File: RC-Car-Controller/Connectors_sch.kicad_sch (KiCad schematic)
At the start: 8 parts, among them J1 Conn_01x02, J4 Conn_01x02, J5 MCU_IF, J6 ANT_IF, J7 2171790001, U2 USBLC6-2SC6

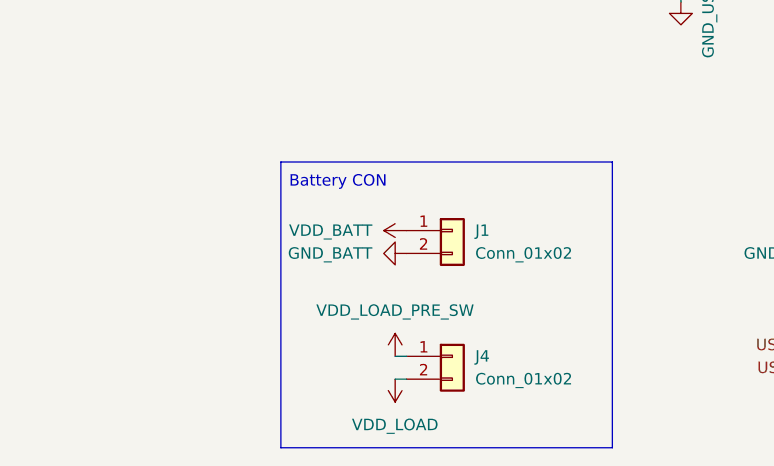
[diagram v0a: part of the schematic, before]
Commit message: Added a switch
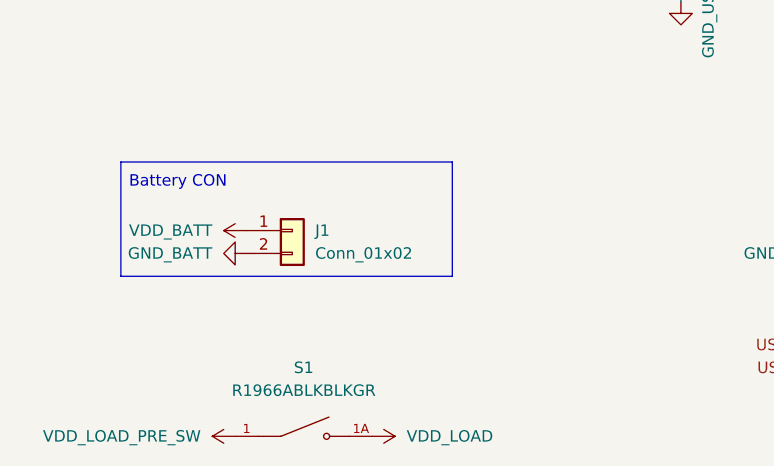
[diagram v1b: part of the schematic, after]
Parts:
- removed J4: Conn_01x02, Connector_JST:JST_XH_B2B-XH-AM_1x02_P2.50mm_Vertical, symbol Connector_Generic:Conn_01x02
- added S1: R1966ABLKBLKGR, R1966ABLKBLKGR:SW_R1966ABLKBLKGR, symbol R1966ABLKBLKGR:R1966ABLKBLKGR
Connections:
- net VDD_LOAD: now also S1.1A
- net VDD_LOAD_PRE_SW: now also S1.1
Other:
- moved on the sheet: J1
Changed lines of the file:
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@@
 		)
 	)
-	(wire
-		(pts
-			(xy 73.66 146.05) (xy 72.39 146.05)
-		)
+	(rectangle
+		(start 41.91 121.92)
+		(end 78.74 134.62)
 		(stroke
 			(width 0)
 			(type default)
 		)
-	)
-	(wire
-		(pts
-			(xy 73.66 143.51) (xy 72.39 143.51)
-		)
-		(stroke
-			(width 0)
-			(type default)
-		)
-	)
-	(rectangle
-		(start 59.69 121.92)
-		(end 96.52 153.67)
-		(stroke
-			(width 0)
-			(type default)
-		)
 		(fill
 			(type none)
@@
 	(text "Battery CON"
 		(exclude_from_sim no)
-		(at 66.04 124.206 0)
+		(at 48.26 124.206 0)
 		(effects
 			(font
@@
 	)
 	(symbol
-		(lib_id "Connector_Generic:Conn_01x02")
-		(at 78.74 143.51 0)
-		(unit 1)
-		(exclude_from_sim no)
-		(in_bom yes)
-		(on_board yes)
-		(dnp no)
-		(fields_autoplaced yes)
-		(property "Reference" "J4"
-			(at 81.28 143.5099 0)
-			(effects
-				(font
-					(size 1.27 1.27)
-				)
-				(justify left)
-			)
-		)
-		(property "Value" "Conn_01x02"
-			(at 81.28 146.0499 0)
-			(effects
-				(font
-					(size 1.27 1.27)
-				)
-				(justify left)
-			)
-		)
-		(property "Footprint" "Connector_JST:JST_XH_B2B-XH-AM_1x02_P2.50mm_Vertical"
-			(at 78.74 143.51 0)
-			(effects
-				(font
-					(size 1.27 1.27)
-				)
-				(hide yes)
-			)
-		)
-		(property "Datasheet" "~"
-			(at 78.74 143.51 0)
-			(effects
-				(font
-					(size 1.27 1.27)
-				)
-				(hide yes)
-			)
-		)
-		(property "Description" "Generic connector, single row, 01x02, script generated (kicad-library-utils/schlib/autogen/connector/)"
-			(at 78.74 143.51 0)
-			(effects
-				(font
-					(size 1.27 1.27)
-				)
-				(hide yes)
-			)
-		)
-		(pin "1"
-		)
-		(pin "2"
-		)
-		(instances
-			(project "RC-Car-Controller"
-				(path "/ba870fd1-751d-4755-8e1a-1ea86ca9e2f6/47812da9-b622-4bda-8507-4e09448e1ff5"
-					(reference "J4")
-					(unit 1)
-				)
-			)
-		)
-	)
-	(symbol
 		(lib_id "power:GND")
 		(at 104.14 104.14 0)
@@
 	(symbol
 		(lib_id "power:+3V3")
-		(at 72.39 146.05 180)
+		(at 69.85 152.4 270)
 		(unit 1)
 		(exclude_from_sim no)
@@
 		(fields_autoplaced yes)
 		(property "Reference" "#PWR013"
-			(at 72.39 142.24 0)
+			(at 66.04 152.4 0)
 			(effects
 				(font
@@
 		)
 		(property "Value" "VDD_LOAD"
-			(at 72.39 151.13 0)
-			(effects
-				(font
-					(size 1.27 1.27)
-				)
+			(at 73.66 152.3999 90)
+			(effects
+				(font
+					(size 1.27 1.27)
+				)
+				(justify left)
 			)
 		)
 		(property "Footprint" ""
-			(at 72.39 146.05 0)
+			(at 69.85 152.4 0)
 			(effects
 				(font
@@
 		)
 		(property "Datasheet" ""
-			(at 72.39 146.05 0)
+			(at 69.85 152.4 0)
 			(effects
 				(font
@@
 		)
 		(property "Description" "Power symbol creates a global label with name \"+3V3\""
-			(at 72.39 146.05 0)
+			(at 69.85 152.4 0)
 			(effects
 				(font
@@
 	)
 	(symbol
+		(lib_id "R1966ABLKBLKGR:R1966ABLKBLKGR")
+		(at 62.23 152.4 0)
+		(unit 1)
+		(exclude_from_sim no)
+		(in_bom yes)
+		(on_board yes)
+		(dnp no)
+		(fields_autoplaced yes)
+		(property "Reference" "S1"
+			(at 62.23 144.78 0)
+			(effects
+				(font
+					(size 1.27 1.27)
+				)
+			)
+		)
+		(property "Value" "R1966ABLKBLKGR"
+			(at 62.23 147.32 0)
+			(effects
+				(font
+					(size 1.27 1.27)
+				)
+			)
+		)
+		(property "Footprint" "R1966ABLKBLKGR:SW_R1966ABLKBLKGR"
+			(at 62.23 152.4 0)
+			(effects
+				(font
+					(size 1.27 1.27)
+				)
+				(justify bottom)
+				(hide yes)
+			)
+		)
+		(property "Datasheet" "https://www.digikey.com/en/products/detail/e-switch/R1966ABLKBLKGR/379042"
+			(at 62.23 152.4 0)
+			(effects
+				(font
+					(size 1.27 1.27)
+				)
+				(hide yes)
+			)
+		)
+		(property "Description" ""
+			(at 62.23 152.4 0)
+			(effects
+				(font
+					(size 1.27 1.27)
+				)
+				(hide yes)
+			)
+		)
+		(property "PARTREV" "E"
+			(at 62.23 152.4 0)
+			(effects
+				(font
+					(size 1.27 1.27)
+				)
+				(justify bottom)
+				(hide yes)
+			)
+		)
+		(property "SNAPEDA_PN" "R1966ABLKBLKGR"
+			(at 62.23 152.4 0)
+			(effects
+				(font
+					(size 1.27 1.27)
+				)
+				(justify bottom)
+				(hide yes)
+			)
+		)
+		(property "STANDARD" "Manufacturer Recommendations"
+			(at 62.23 152.4 0)
+			(effects
+				(font
+					(size 1.27 1.27)
+				)
+				(justify bottom)
+				(hide yes)
+			)
+		)
+		(property "MAXIMUM_PACKAGE_HEIGHT" "14.8 mm"
+			(at 62.23 152.4 0)
+			(effects
+				(font
+					(size 1.27 1.27)
+				)
+				(justify bottom)
+				(hide yes)
+			)
+		)
+		(property "MANUFACTURER" "E-Switch"
+			(at 62.23 152.4 0)
+			(effects
+				(font
+					(size 1.27 1.27)
+				)
+				(justify bottom)
+				(hide yes)
+			)
+		)
+		(pin "1"
+		)
+		(pin "1A"
+		)
+		(instances
+			(project ""
+				(path "/ba870fd1-751d-4755-8e1a-1ea86ca9e2f6/47812da9-b622-4bda-8507-4e09448e1ff5"
+					(reference "S1")
+					(unit 1)
+				)
+			)
+		)
+	)
+	(symbol
 		(lib_id "power:GND")
 		(at 121.92 81.28 0)
@@
 	(symbol
 		(lib_id "power:+3V3")
-		(at 72.39 143.51 0)
+		(at 54.61 152.4 90)
 		(unit 1)
 		(exclude_from_sim no)
@@
 		(fields_autoplaced yes)
 		(property "Reference" "#PWR096"
-			(at 72.39 147.32 0)
+			(at 58.42 152.4 0)
 			(effects
 				(font
@@
 		)
 		(property "Value" "VDD_LOAD_PRE_SW"
-			(at 72.39 138.43 0)
-			(effects
-				(font
-					(size 1.27 1.27)
-				)
+			(at 50.8 152.3999 90)
+			(effects
+				(font
+					(size 1.27 1.27)
+				)
+				(justify left)
 			)
 		)
 		(property "Footprint" ""
-			(at 72.39 143.51 0)
+			(at 54.61 152.4 0)
 			(effects
 				(font
@@
 		)
 		(property "Datasheet" ""
-			(at 72.39 143.51 0)
+			(at 54.61 152.4 0)
 			(effects
 				(font
@@
 		)
 		(property "Description" "Power symbol creates a global label with name \"+3V3\""
-			(at 72.39 143.51 0)
+			(at 54.61 152.4 0)
 			(effects
 				(font
@@
 	(symbol
 		(lib_id "Connector_Generic:Conn_01x02")
-		(at 78.74 129.54 0)
+		(at 60.96 129.54 0)
 		(unit 1)
 		(exclude_from_sim no)
@@
 		(fields_autoplaced yes)
 		(property "Reference" "J1"
-			(at 81.28 129.5399 0)
+			(at 63.5 129.5399 0)
 			(effects
 				(font
@@
 		)
 		(property "Value" "Conn_01x02"
-			(at 81.28 132.0799 0)
+			(at 63.5 132.0799 0)
 			(effects
 				(font
@@
 		)
 		(property "Footprint" "Connector_JST:JST_XH_B2B-XH-AM_1x02_P2.50mm_Vertical"
-			(at 78.74 129.54 0)
+			(at 60.96 129.54 0)
 			(effects
 				(font
@@
 		)
 		(property "Datasheet" "~"
-			(at 78.74 129.54 0)
+			(at 60.96 129.54 0)
 			(effects
 				(font
@@
 		)
 		(property "Description" "Generic connector, single row, 01x02, script generated (kicad-library-utils/schlib/autogen/connector/)"
-			(at 78.74 129.54 0)
+			(at 60.96 129.54 0)
 			(effects
 				(font
@@
 	(symbol
 		(lib_id "power:+3V3")
-		(at 73.66 129.54 90)
+		(at 55.88 129.54 90)
 		(unit 1)
 		(exclude_from_sim no)
@@
 		(fields_autoplaced yes)
 		(property "Reference" "#PWR092"
-			(at 77.47 129.54 0)
+			(at 59.69 129.54 0)
 			(effects
 				(font
@@
 		)
 		(property "Value" "VDD_BATT"
-			(at 69.85 129.5399 90)
+			(at 52.07 129.5399 90)
 			(effects
 				(font
@@
 		)
 		(property "Footprint" ""
-			(at 73.66 129.54 0)
+			(at 55.88 129.54 0)
 			(effects
 				(font
@@
 		)
 		(property "Datasheet" ""
-			(at 73.66 129.54 0)
+			(at 55.88 129.54 0)
 			(effects
 				(font
@@
 		)
 		(property "Description" "Power symbol creates a global label with name \"+3V3\""
-			(at 73.66 129.54 0)
+			(at 55.88 129.54 0)
 			(effects
 				(font
@@
 	(symbol
 		(lib_id "power:GND")
-		(at 73.66 132.08 270)
+		(at 55.88 132.08 270)
 		(unit 1)
 		(exclude_from_sim no)
@@
 		(fields_autoplaced yes)
 		(property "Reference" "#PWR093"
-			(at 67.31 132.08 0)
+			(at 49.53 132.08 0)
 			(effects
 				(font
@@
 		)
 		(property "Value" "GND_BATT"
-			(at 69.85 132.0799 90)
+			(at 52.07 132.0799 90)
 			(effects
 				(font
@@
 		)
 		(property "Footprint" ""
-			(at 73.66 132.08 0)
+			(at 55.88 132.08 0)
 			(effects
 				(font
@@
 		)
 		(property "Datasheet" ""
-			(at 73.66 132.08 0)
+			(at 55.88 132.08 0)
 			(effects
 				(font
@@
 		)
 		(property "Description" "Power symbol creates a global label with name \"GND\" , ground"
-			(at 73.66 132.08 0)
-			(effects
-				(font
+			(at 55.88 132.08 0)
+			(effects
+				(font

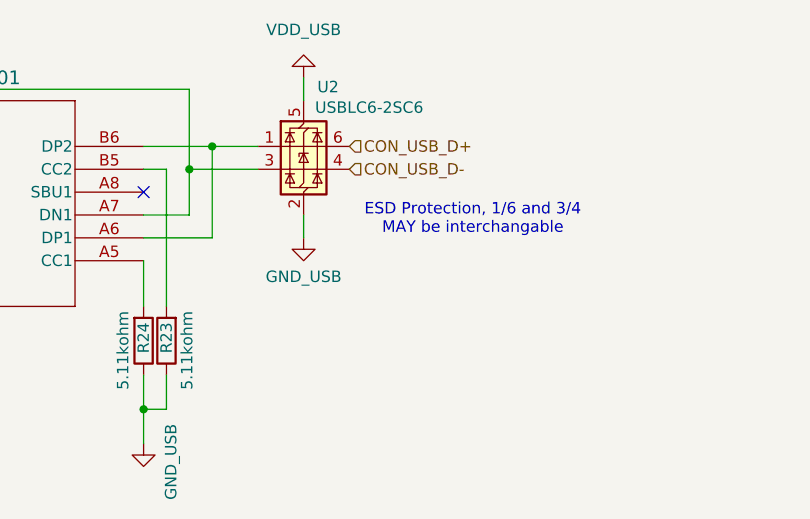
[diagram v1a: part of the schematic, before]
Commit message: Did power schtuff
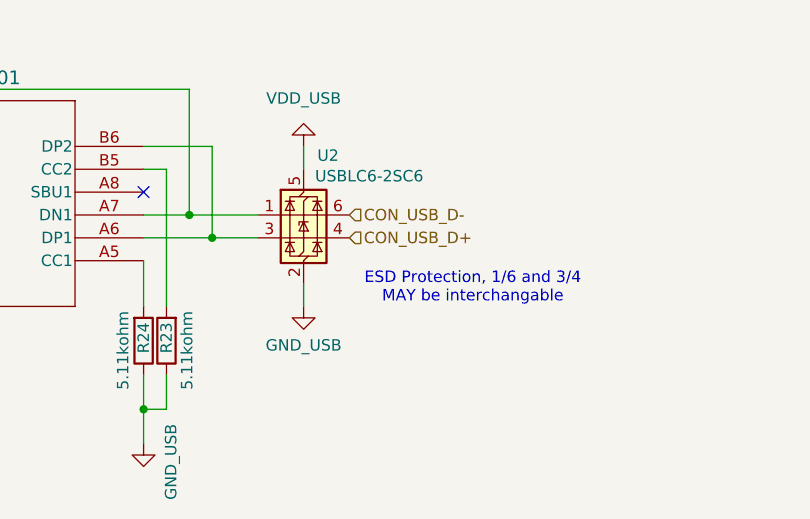
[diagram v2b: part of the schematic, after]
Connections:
- net CON_USB_D+: now also U2.4 (I/O2); no longer U2.6 (I/O1)
- net CON_USB_D-: now also U2.6 (I/O1); no longer U2.4 (I/O2)
- net at J7.A6 (DP1), J7.B6 (DP2): now also U2.3 (I/O2); no longer U2.1 (I/O1)
- net at J7.A7 (DN1), J7.B7 (DN2): now also U2.1 (I/O1); no longer U2.3 (I/O2)
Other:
- moved on the sheet: U2
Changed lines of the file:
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@@
 	(paper "A4")
 	(junction
-		(at 111.76 71.12)
+		(at 111.76 81.28)
 		(diameter 0)
 		(color 0 0 0 0)
@@
 	)
 	(junction
-		(at 109.22 73.66)
+		(at 109.22 78.74)
 		(diameter 0)
 		(color 0 0 0 0)
@@
 	(wire
 		(pts
-			(xy 111.76 71.12) (xy 116.84 71.12)
-		)
-		(stroke
-			(width 0)
-			(type default)
-		)
-	)
-	(wire
-		(pts
 			(xy 104.14 83.82) (xy 104.14 88.9)
 		)
@@
 	(wire
 		(pts
-			(xy 109.22 78.74) (xy 109.22 73.66)
+			(xy 109.22 64.77) (xy 109.22 78.74)
 		)
 		(stroke
@@
 	(wire
 		(pts
-			(xy 109.22 73.66) (xy 116.84 73.66)
-		)
-		(stroke
-			(width 0)
-			(type default)
-		)
-	)
-	(wire
-		(pts
 			(xy 60.96 81.28) (xy 63.5 81.28)
 		)
@@
 	(wire
 		(pts
-			(xy 109.22 73.66) (xy 109.22 64.77)
-		)
-		(stroke
-			(width 0)
-			(type default)
-		)
-	)
-	(wire
-		(pts
 			(xy 104.14 78.74) (xy 109.22 78.74)
 		)
@@
 	(wire
 		(pts
-			(xy 121.92 63.5) (xy 121.92 66.04)
-		)
-		(stroke
-			(width 0)
-			(type default)
-		)
-	)
-	(wire
-		(pts
-			(xy 121.92 81.28) (xy 121.92 78.74)
+			(xy 121.92 71.12) (xy 121.92 73.66)
+		)
+		(stroke
+			(width 0)
+			(type default)
+		)
+	)
+	(wire
+		(pts
+			(xy 121.92 88.9) (xy 121.92 86.36)
+		)
+		(stroke
+			(width 0)
+			(type default)
+		)
+	)
+	(wire
+		(pts
+			(xy 111.76 81.28) (xy 116.84 81.28)
 		)
 		(stroke
@@
 		(pts
 			(xy 60.96 71.12) (xy 63.5 71.12)
+		)
+		(stroke
+			(width 0)
+			(type default)
+		)
+	)
+	(wire
+		(pts
+			(xy 109.22 78.74) (xy 116.84 78.74)
 		)
 		(stroke
@@
 	(text "ESD Protection, 1/6 and 3/4 \nMAY be interchangable"
 		(exclude_from_sim no)
-		(at 140.716 79.248 0)
+		(at 140.716 86.868 0)
 		(effects
 			(font
@@
 	(hierarchical_label "CON_USB_D-"
 		(shape input)
-		(at 127 73.66 0)
+		(at 127 78.74 0)
 		(fields_autoplaced yes)
 		(effects
@@
 	(hierarchical_label "CON_USB_D+"
 		(shape input)
-		(at 127 71.12 0)
+		(at 127 81.28 0)
 		(fields_autoplaced yes)
 		(effects
@@
 	(symbol
 		(lib_id "Power_Protection:USBLC6-2SC6")
-		(at 121.92 71.12 0)
+		(at 121.92 78.74 0)
 		(unit 1)
 		(exclude_from_sim no)
@@
 		(dnp no)
 		(property "Reference" "U2"
-			(at 123.444 64.516 0)
+			(at 123.444 72.136 0)
 			(effects
 				(font
@@
 		)
 		(property "Value" "USBLC6-2SC6"
-			(at 123.19 66.802 0)
+			(at 123.19 74.422 0)
 			(effects
 				(font
@@
 		)
 		(property "Footprint" "Package_TO_SOT_SMD:SOT-23-6"
-			(at 123.19 77.47 0)
+			(at 123.19 85.09 0)
 			(effects
 				(font
@@
 		)
 		(property "Datasheet" "https://www.digikey.ca/en/products/detail/stmicroelectronics/USBLC6-2SC6/1040559"
-			(at 123.19 79.375 0)
+			(at 123.19 86.995 0)
 			(effects
 				(font
@@
 		)
 		(property "Description" "Very low capacitance ESD protection diode, 2 data-line, SOT-23-6"
-			(at 121.92 71.12 0)
+			(at 121.92 78.74 0)
 			(effects
 				(font
@@
 	(symbol
 		(lib_id "power:GND")
-		(at 121.92 81.28 0)
+		(at 121.92 88.9 0)
 		(unit 1)
 		(exclude_from_sim no)
@@
 		(dnp no)
 		(property "Reference" "#PWR043"
-			(at 121.92 87.63 0)
+			(at 121.92 95.25 0)
 			(effects
 				(font
@@
 		)
 		(property "Value" "GND_USB"
-			(at 121.92 85.598 0)
+			(at 121.92 93.218 0)
 			(effects
 				(font
@@
 		)
 		(property "Footprint" ""
-			(at 121.92 81.28 0)
+			(at 121.92 88.9 0)
 			(effects
 				(font
@@
 		)
 		(property "Datasheet" ""
-			(at 121.92 81.28 0)
+			(at 121.92 88.9 0)
 			(effects
 				(font
@@
 		)
 		(property "Description" "Power symbol creates a global label with name \"GND\" , ground"
-			(at 121.92 81.28 0)
+			(at 121.92 88.9 0)
 			(effects
 				(font
@@
 	(symbol
 		(lib_id "power:GND")
-		(at 121.92 63.5 180)
+		(at 121.92 71.12 180)
 		(unit 1)
 		(exclude_from_sim no)
@@
 		(dnp no)
 		(property "Reference" "#PWR042"
-			(at 121.92 57.15 0)
+			(at 121.92 64.77 0)
 			(effects
 				(font
@@
 		)
 		(property "Value" "VDD_USB"
-			(at 121.92 58.166 0)
+			(at 121.92 65.786 0)
 			(effects
 				(font
@@
 		)
 		(property "Footprint" ""
-			(at 121.92 63.5 0)
+			(at 121.92 71.12 0)
 			(effects
 				(font
@@
 		)
 		(property "Datasheet" ""
-			(at 121.92 63.5 0)
+			(at 121.92 71.12 0)
 			(effects
 				(font
@@
 		)
 		(property "Description" "Power symbol creates a global label with name \"GND\" , ground"
-			(at 121.92 63.5 0)
-			(effects
-				(font
+			(at 121.92 71.12 0)
+			(effects
+				(font
